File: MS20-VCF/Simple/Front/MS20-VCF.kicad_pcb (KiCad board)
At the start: 2 copper layers, 60 x 130 mm, 4 parts

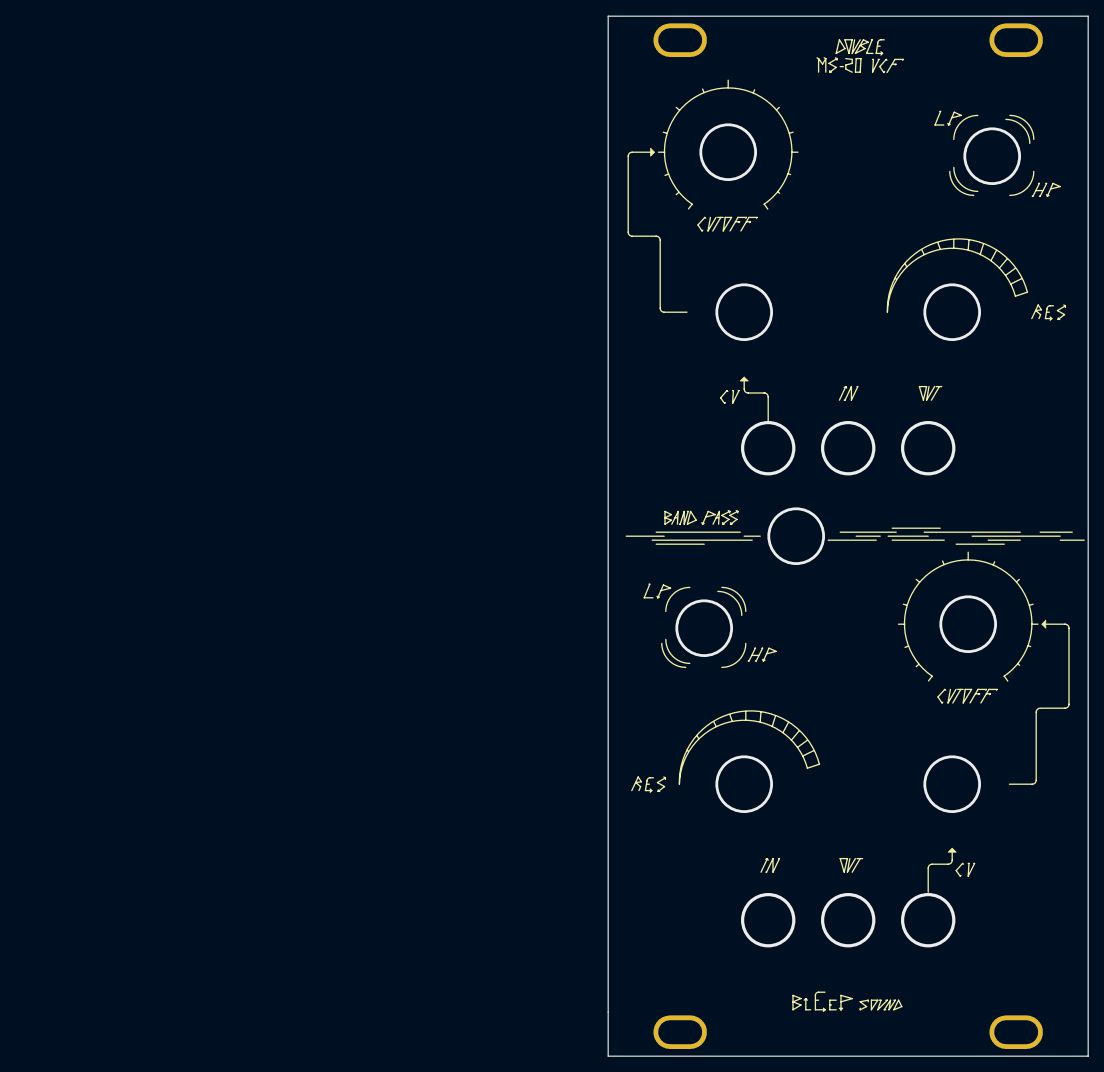
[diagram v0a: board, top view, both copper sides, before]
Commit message: update gerber
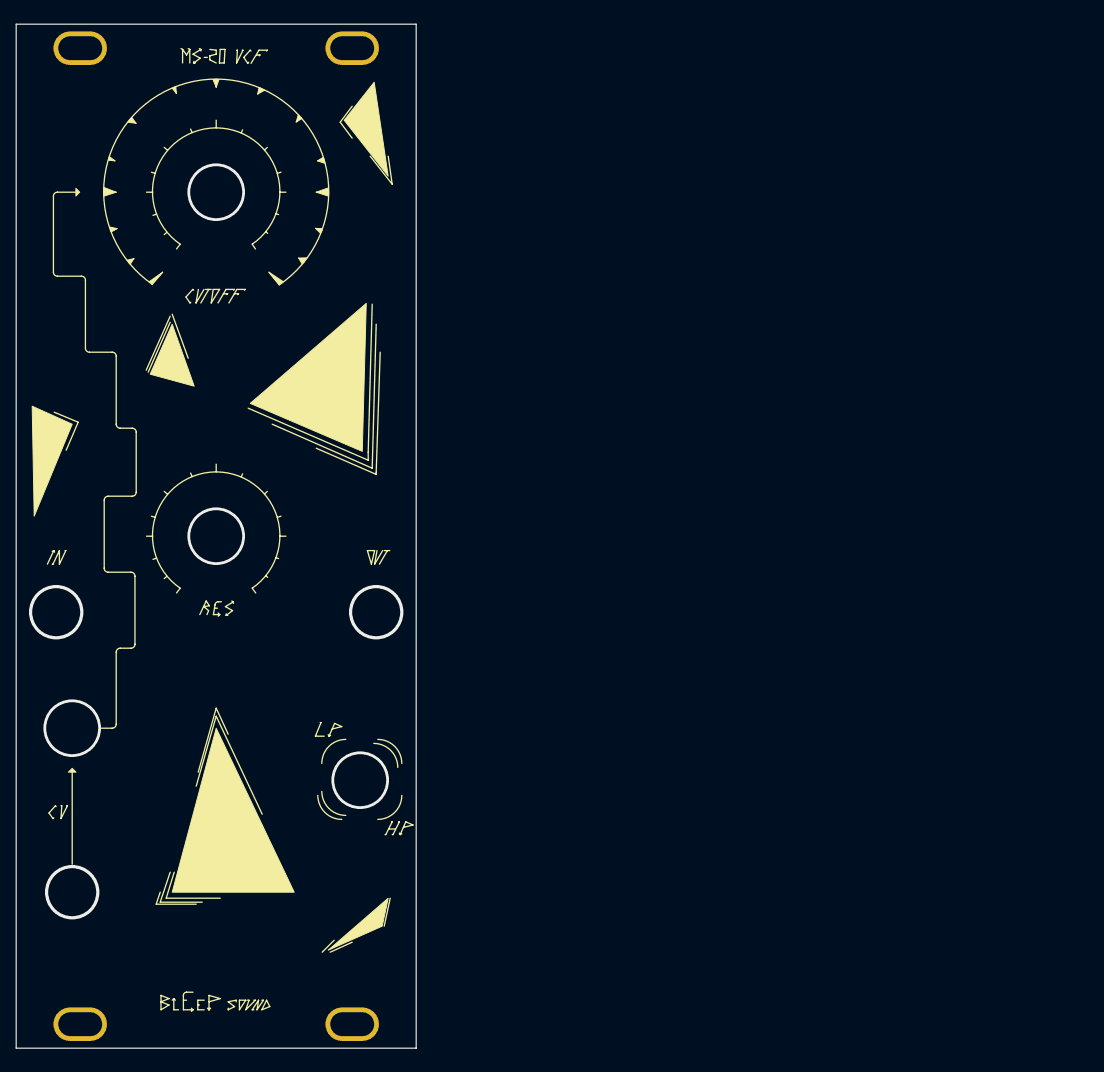
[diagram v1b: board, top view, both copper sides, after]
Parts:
- moved H2 83.0 mm to (145.0, 30.5)
- moved H3 83.0 mm to (145.0, 152.5)
- moved H1 75.0 mm to (111.0, 30.5)
- moved H4 75.0 mm to (111.0, 152.5)
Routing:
- net GND: vias 15 -> 7
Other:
- board size 60 x 130 mm -> 50 x 128 mm
- board text added: "MS-20 VCF Face plate V1.0 BleepSound 2022"
